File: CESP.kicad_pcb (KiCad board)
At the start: 2 copper layers, 55.9 x 44.7 mm, 9 parts

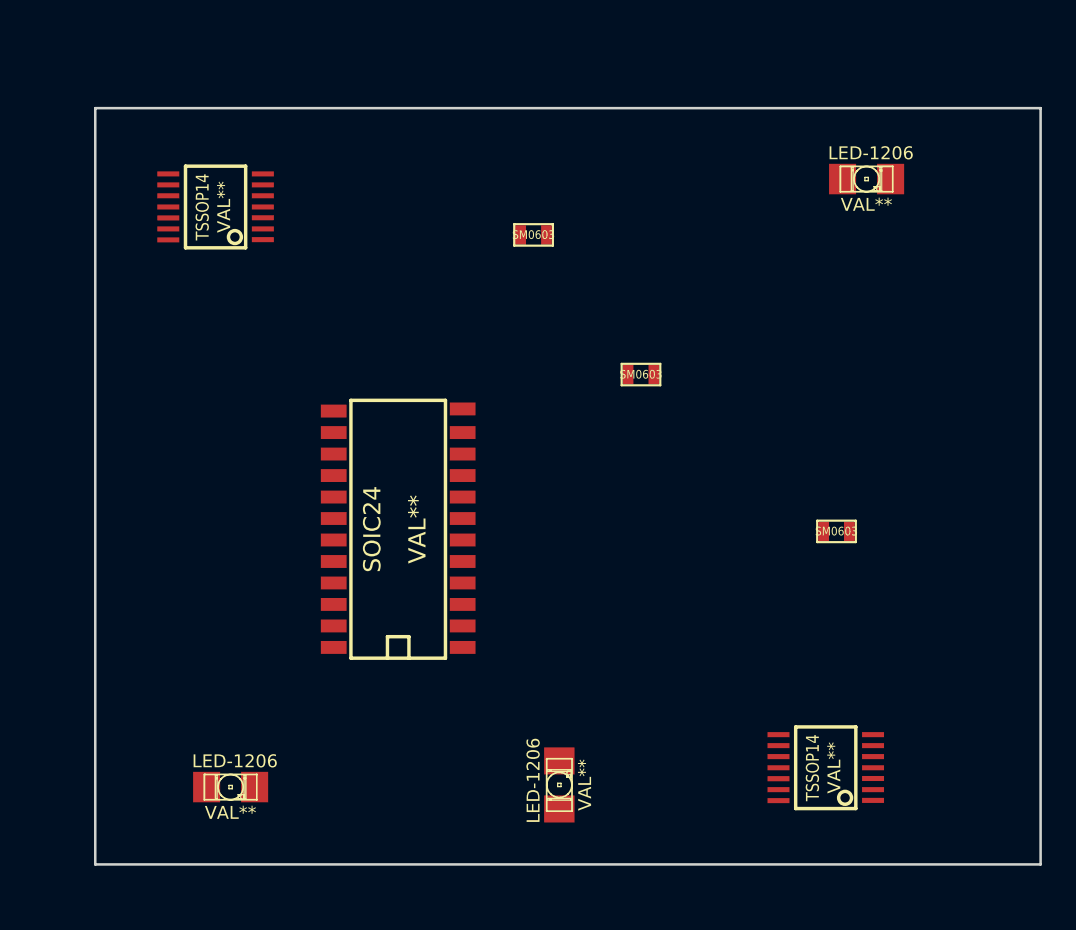
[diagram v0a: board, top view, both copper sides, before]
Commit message: no message
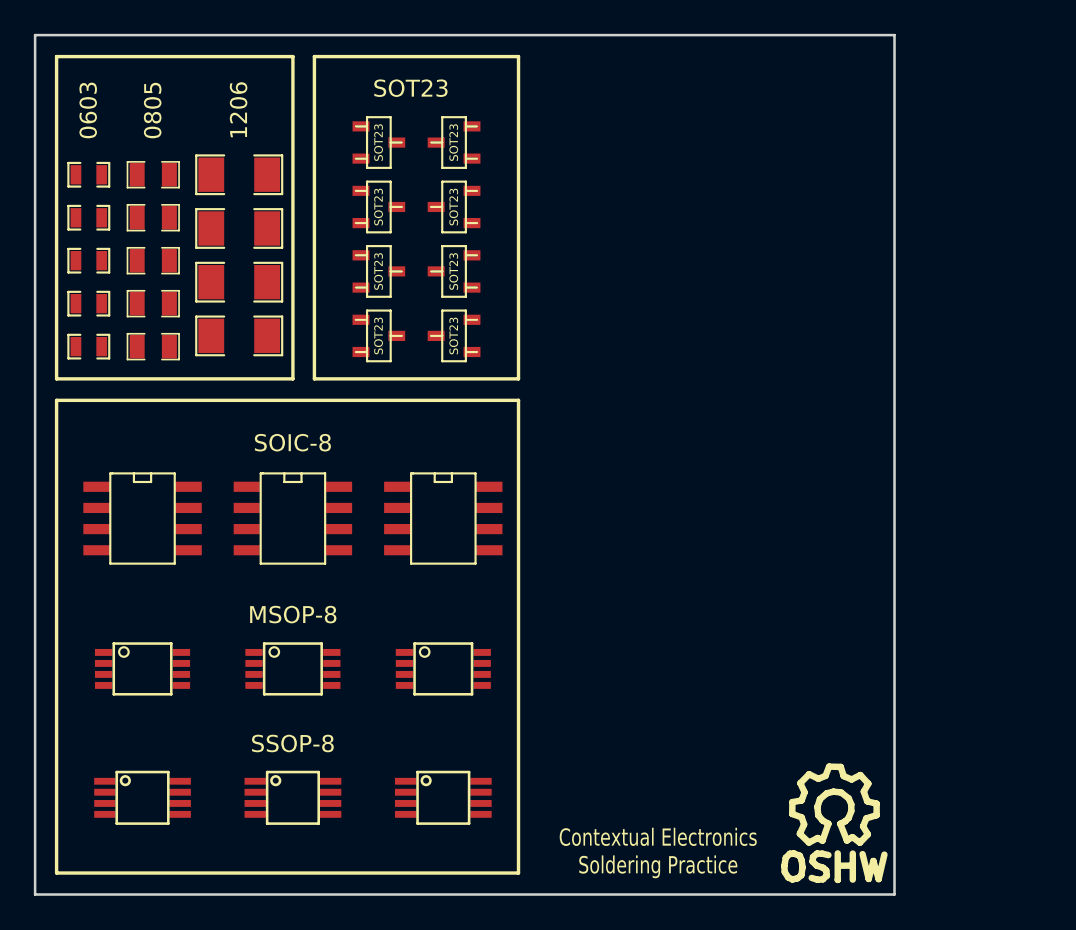
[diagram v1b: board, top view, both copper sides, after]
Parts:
- removed LED-1206 (x3): VAL**, LED-1206
- removed SM0603 (x3): Val**, SM0603
- removed SOIC24: VAL**, SOIC24
- removed TSSOP14 (x2): VAL**, TSSOP14
- added MSOP-8: U***, SSOP_Packages:MSOP-8, F.Cu at (176.5, 128.9)
- added MSOP-8: U***, SSOP_Packages:MSOP-8, F.Cu at (167.6, 128.9)
- added MSOP-8: U***, SSOP_Packages:MSOP-8, F.Cu at (158.8, 128.9)
- added SM0603_resistor: Val**, SMD_Packages:SM0603_Resistor, F.Cu at (155.6, 99.7)
- added SM0603_resistor: Val**, SMD_Packages:SM0603_Resistor, F.Cu at (155.6, 102.2)
- added SM0603_resistor: Val**, SMD_Packages:SM0603_Resistor, F.Cu at (155.6, 104.8)
- added SM0603_resistor: Val**, SMD_Packages:SM0603_Resistor, F.Cu at (155.6, 107.3)
- added SM0603_resistor: Val**, SMD_Packages:SM0603_Resistor, F.Cu at (155.6, 109.9)
- added SM0805: Val*, SMD_Packages:SM0805, F.Cu at (159.4, 109.9)
- added SM0805: Val*, SMD_Packages:SM0805, F.Cu at (159.4, 107.3)
- added SM0805: Val*, SMD_Packages:SM0805, F.Cu at (159.4, 104.8)
- added SM0805: Val*, SMD_Packages:SM0805, F.Cu at (159.4, 102.2)
- added SM0805: Val*, SMD_Packages:SM0805, F.Cu at (159.4, 99.7)
- added SM1206: Val**, SMD_Packages:SM1206, F.Cu at (164.5, 99.7)
- added SM1206: Val**, SMD_Packages:SM1206, F.Cu at (164.5, 102.9)
- added SM1206: Val**, SMD_Packages:SM1206, F.Cu at (164.5, 106.0)
- added SM1206: Val**, SMD_Packages:SM1206, F.Cu at (164.5, 109.2)
- added SOIC-8: VAL**, SOIC_Packages:SOIC-8_N, F.Cu at (158.8, 120.0)
- added SOIC-8_N: VAL**, SOIC_Packages:SOIC-8_N, F.Cu at (167.6, 120.0)
- added SOIC-8_N: VAL**, SOIC_Packages:SOIC-8_N, F.Cu at (176.5, 120.0)
- added SOT23: Q***, Transistors_SMD:sot23, F.Cu at (172.7, 97.8)
- added SOT23: Q***, Transistors_SMD:sot23, F.Cu at (177.2, 97.8)
- added SOT23: Q***, Transistors_SMD:sot23, F.Cu at (177.2, 101.6)
- added SOT23: Q***, Transistors_SMD:sot23, F.Cu at (172.7, 101.6)
- added SOT23: Q***, Transistors_SMD:sot23, F.Cu at (172.7, 105.4)
- added SOT23: Q***, Transistors_SMD:sot23, F.Cu at (172.7, 109.2)
- added SOT23: Q***, Transistors_SMD:sot23, F.Cu at (177.2, 105.4)
- added SOT23: Q***, Transistors_SMD:sot23, F.Cu at (177.2, 109.2)
- added SSOP-8: Val**, SSOP_Packages:SSOP-8, F.Cu at (176.5, 136.5)
- added SSOP-8: Val**, SSOP_Packages:SSOP-8, F.Cu at (167.6, 136.5)
- added SSOP-8: Val**, SSOP_Packages:SSOP-8, F.Cu at (158.8, 136.5)
- added SYM: Symbol_OSHW-Logo_SilkScreen_07Jul2012, Footprint_Symbols:Symbol_OSHW-Logo_SilkScreen_07Jul2012, F.Cu at (199.6, 137.2)
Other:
- board size 55.9 x 44.7 mm -> 50.8 x 50.8 mm
- board text added: "0603"
- board text added: "0805"
- board text added: "1206"
- board text added: "Contextual Electronics Soldering Practice"
- board text added: "MSOP-8"
- board text added: "SOIC-8"
- board text added: "SOT23"
- board text added: "SSOP-8"
- board text removed: "NOTE: THIS IS JUST A TEST BOARD REMOVE ALL COMPONENTS AND CREATE YOUR OWN INCLUDE SCHEMATIC HOOKUPS/NETLIST"
